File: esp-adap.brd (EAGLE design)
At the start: 27.9 x 14.9 mm, 3 parts

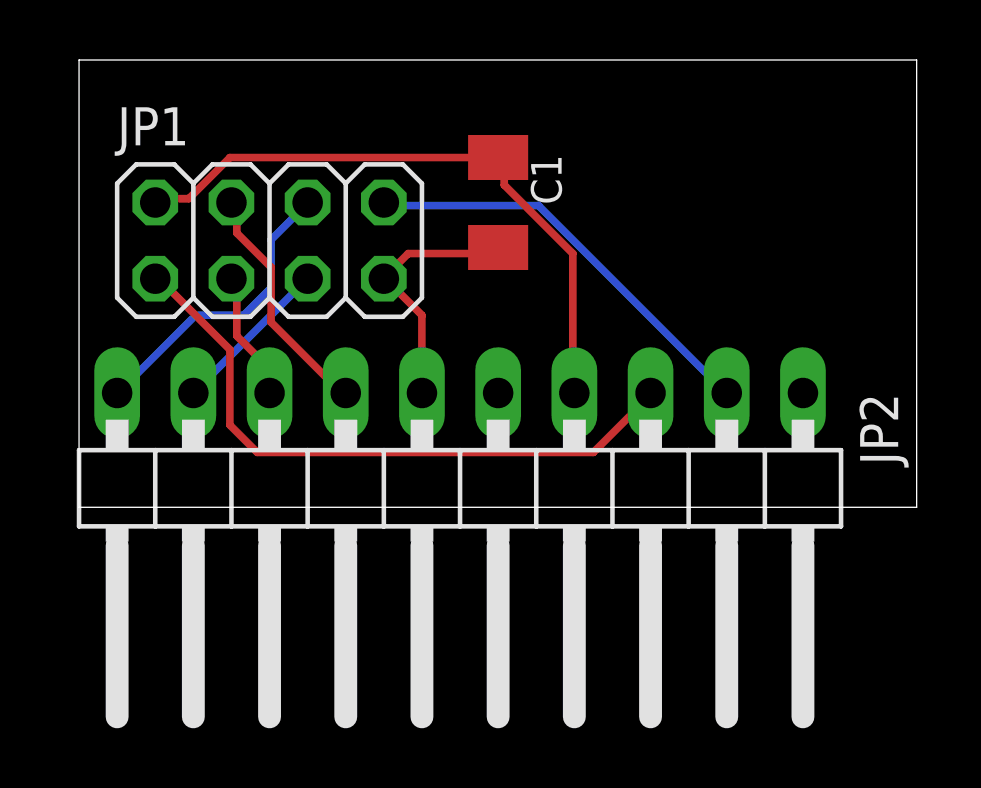
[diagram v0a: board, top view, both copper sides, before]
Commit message: board done
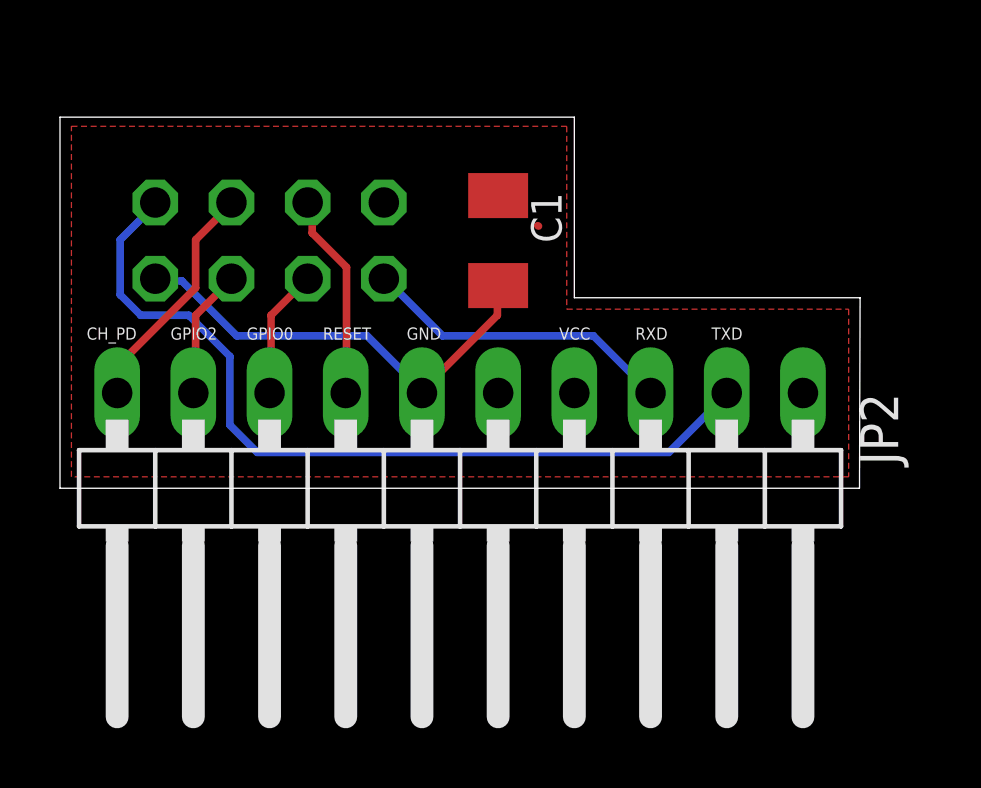
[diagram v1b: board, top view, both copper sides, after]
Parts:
- moved C1 1.27 mm to (14.0, 8.89)
- flipped JP1 to the bottom
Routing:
- net VCC: track 21.0 -> 0.00 mm
- net TXD: track 14.0 -> 28.1 mm
- net RXD: track 21.2 -> 10.5 mm
- net GND: track 8.70 -> 15.1 mm
- net CH_PD: track 9.92 -> 7.93 mm
- net RESET: track 8.01 -> 6.91 mm
- net GPIO2: track 5.39 -> 4.33 mm
- added copper zone on layer 1, net VCC
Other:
- board size 27.9 x 14.9 mm -> 26.7 x 12.4 mm
- board text added: "CH_PD"
- board text added: "GND"
- board text added: "GPIO0"
- board text added: "GPIO2"
- board text added: "RESET"
- board text added: "RXD"
- board text added: "TXD"
- board text added: "VCC"
- board text added: "github.com/fu0x11/esp8266-breadboard-adapter"
